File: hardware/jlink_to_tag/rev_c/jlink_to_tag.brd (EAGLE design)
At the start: 25.9 x 33 mm, 12 parts, among them J2 JLINK_6PIN_TAG-CON, U1 LT1763CS8-3.3

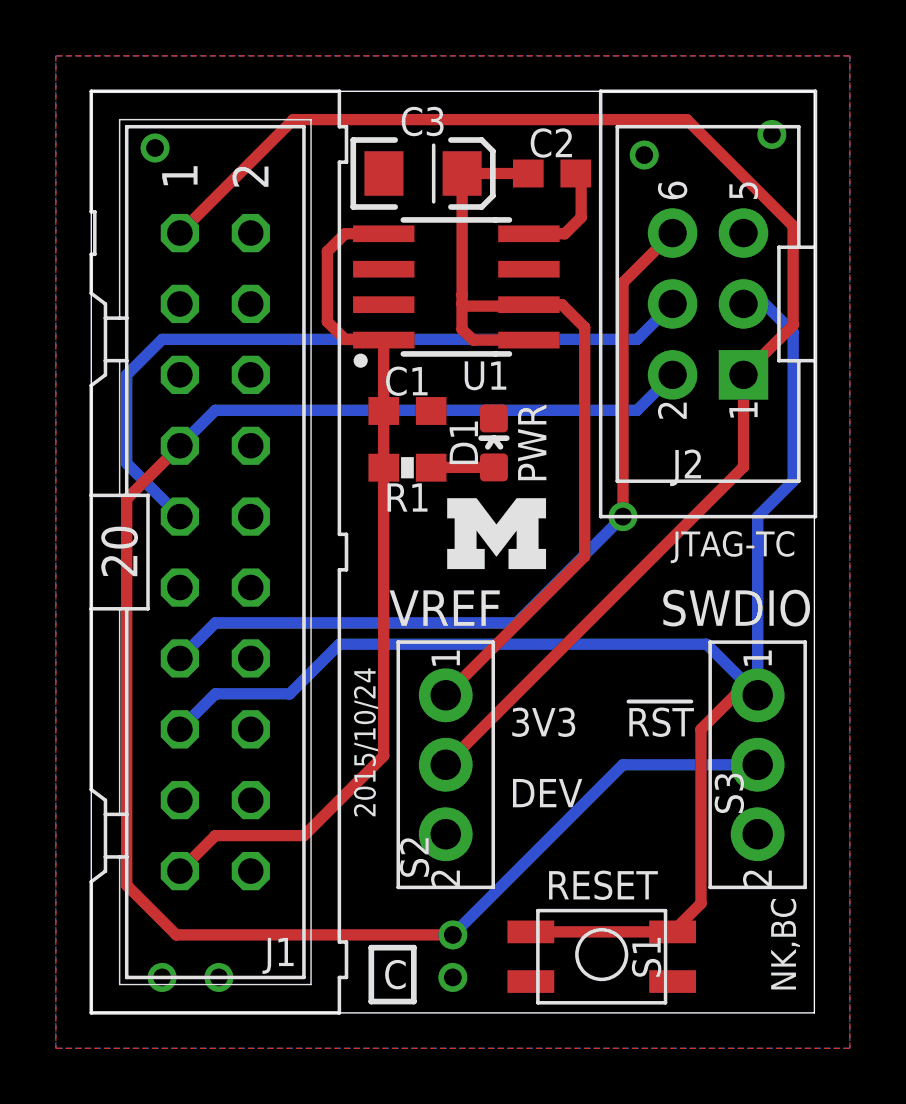
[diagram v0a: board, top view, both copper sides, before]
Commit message: 1x1.3 inches
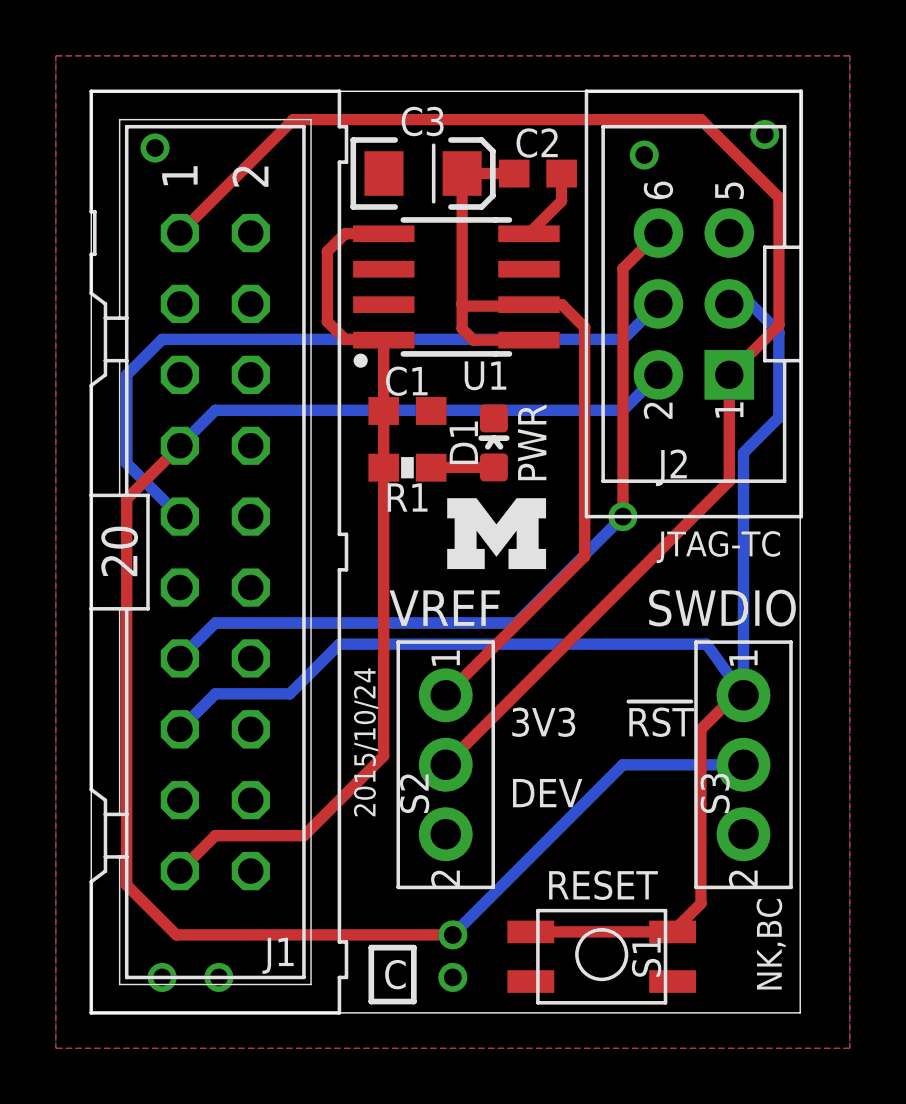
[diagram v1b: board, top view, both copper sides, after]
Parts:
- moved C2 0.51 mm to (16.0, 30.1)
- moved S3 0.51 mm to (23.4, 8.89)
- moved J2 0.51 mm to (21.6, 25.4)
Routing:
- net N$4: track 3.77 -> 2.64 mm
- net SWDIO/TMS: track 61.1 -> 60.1 mm
- net NRESET: track 53.7 -> 52.9 mm
- net 3V3: track 30.5 -> 30.0 mm
- net SWCLK/TCK: track 26.5 -> 26.0 mm
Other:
- board size 25.9 x 33 mm -> 25.4 x 33 mm
